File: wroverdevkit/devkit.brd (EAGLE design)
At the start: 33 x 59.4 mm, 42 parts, among them IC1 FT231XQ, Q3 BSS138, Q4 BSS138, T1 TRANSISTORMMBT2222, T2 TRANSISTORMMBT2222, T3 TRANSISTORMMBT2222

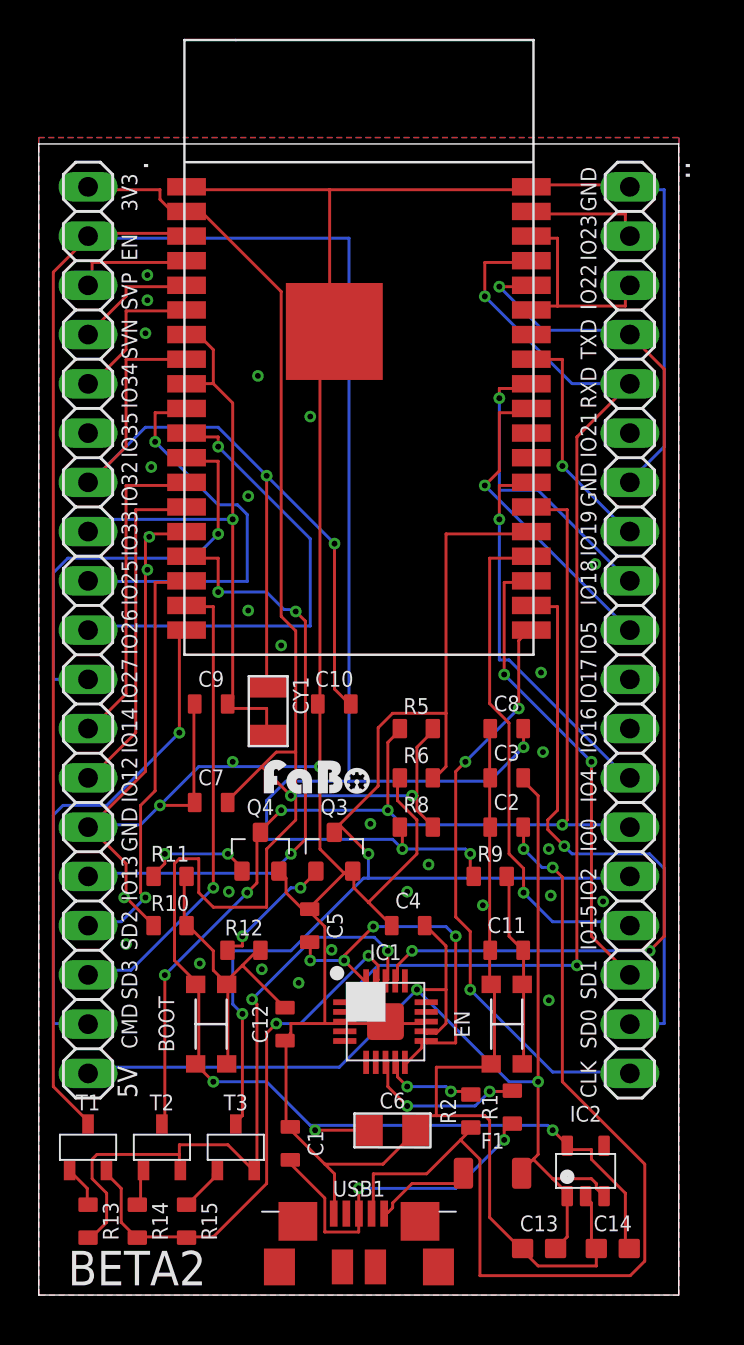
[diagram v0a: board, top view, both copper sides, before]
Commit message: devボード見直し
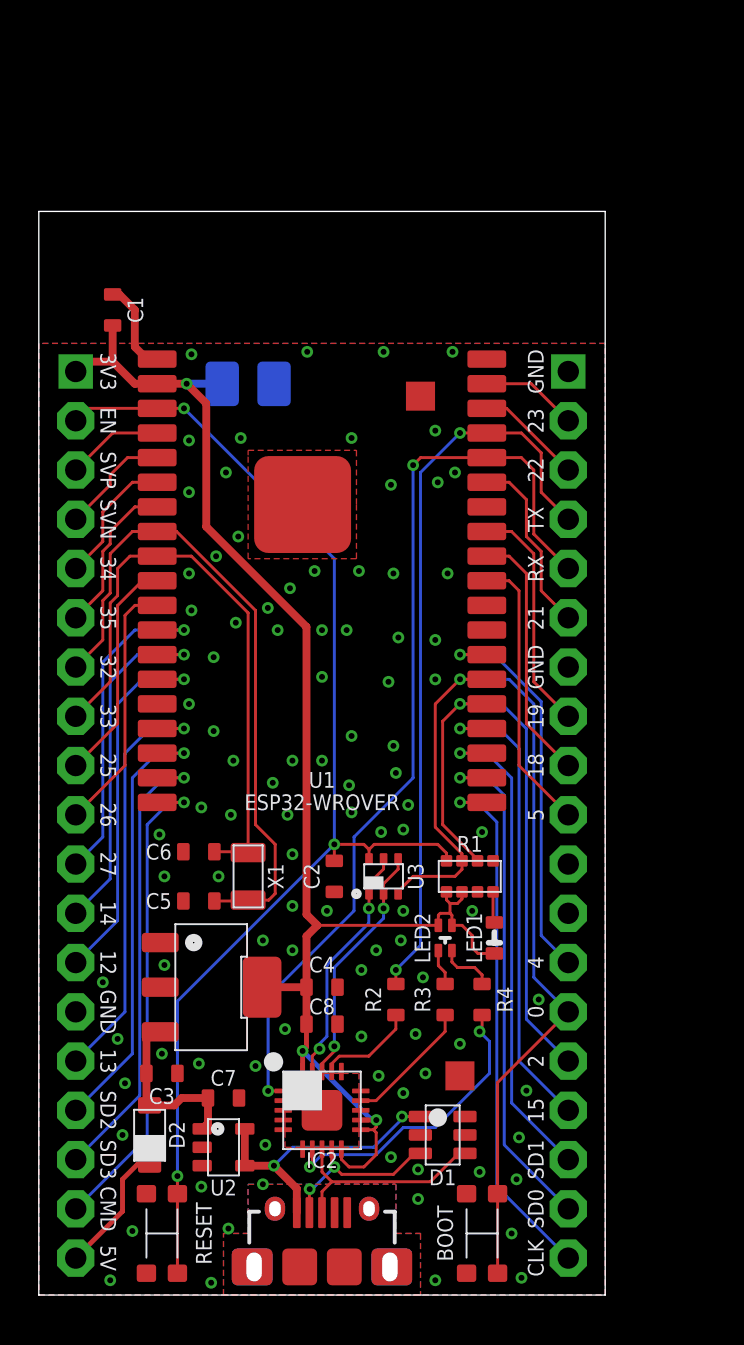
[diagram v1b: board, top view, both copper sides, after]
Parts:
- removed ., ..: (no value), pinhead:1X19
- removed C10, C9: 27pf, FaBo-Capacitor:0603-NARROW
- removed C11, C12: 1nf, FaBo-Capacitor:0603-NARROW
- removed C13, C14: 1uF, FaBo-Capacitor:0603
- removed CY1: CRYSTALABS07, FaBo-Crystal:ABRACOM-ABS07-32.768KHZ
- removed EN: (no value), FaBo-Switch:KMR2
- removed F1: (no value), FaBo-Parts:NANOSMDC035F
- removed Q3, Q4: BSS138, FaBo-etc:SOT23-3
- removed R10: 10K, FaBo-Resistors:0603-NARROW
- removed R11, R12: 1K, FaBo-Resistors:0603-NARROW
- removed R13, R14, R15: 100K, FaBo-Resistors:0603-NARROW
- removed R5, R6: 5K, FaBo-Resistors:0603-NARROW
- removed R8: 12K, FaBo-Resistors:0603-NARROW
- removed R9: 470, FaBo-Resistors:0603-NARROW
- removed T1, T2, T3: TRANSISTORMMBT2222, FaBo-Transistor:SOT-23
- removed U$1: ESP32-WROVER, FaBo-ESP32:ESP32-WROVER
- removed U$3: (no value), FaBo-Logo:LOGO_FABO_S
- added C0: NP, component:MULTIPAD0603
- added CN1, CN2: (no value), component:PIN_1X19
- added D1: ESDA6V1BC6, component:SOT-23-6L
- added D2: (no value), component:SOD-123FL_RB161MM-20
- added FID1, FID2: FIDUCIAL-TOP, component:FIDUCIAL_15_TOP
- added LED1: (no value), component:LED_0603
- added LED2: (no value), component:HSMF-C16X
- added LOGO1: (no value), component:LOGO_FABO_M_BOTTOM
- added R3, R4: 1k, component:EIA0603
- added RESET: (no value), component:KMR2-TACT
- added U1: (no value), component:ESP32-WROVER-B
- added U2: TPS2065DBVR, component:SOT-23-5
- added U3: BS138PS, component:SOT-363
- added X1: 32.768k, component:ABS07
- BOOT: device FaBo-Switch:KMR2 -> component:KMR2-TACT
- C1: value 47pF -> 0.1uF; device FaBo-Capacitor:0603-NARROW -> component:EIA0603
- C2: value 47pF -> 0.01uF; device FaBo-Capacitor:0603-NARROW -> component:EIA0603
- C3: value 0.1uF -> 1uF; device FaBo-Capacitor:0603-NARROW -> component:EIA0603
- C4: value 4.7uF -> 1uF; device FaBo-Capacitor:0603-NARROW -> component:EIA0603
- C5: value 0.1uF -> 4.3pF; device FaBo-Capacitor:0603-NARROW -> component:EIA0603
- C6: value 100uF -> 4.3pF; device FaBo-Capacitor:1206 -> component:EIA0603
- C7: value 1uf -> 10uF; device FaBo-Capacitor:0603-NARROW -> component:EIA0603
- C8: value 0.1uf -> 0.1uF; device FaBo-Capacitor:0603-NARROW -> component:EIA0603
- IC1: value FT231XQ -> ADP3338AKCZ-3.3; device FaBo-USB:QFN-20_FT231X -> component:SOT-223-KC3
- IC2: value (none) -> FT231XQ; device FaBo-Supply:SOT-23-5 -> component:QFN-20
- R1: value 27 -> 10k; device FaBo-Resistors:0603-NARROW -> component:EXBV8V
- R2: value 27 -> 470; device FaBo-Resistors:0603-NARROW -> component:EIA0603
- USB1: value (none) -> ZX62D-B-5PA8(30); device FaBo-USB:ZX62R-B-5P -> component:ZX62D-B-5PA8
- moved C1 43.9 mm to (3.81, 50.8)
- moved C3 23.4 mm to (6.35, 11.4), turned to 180 degrees
- moved C8 18.0 mm to (14.6, 14.0), turned to 180 degrees
- moved BOOT 17.7 mm to (22.9, 3.17)
- moved C6 17.5 mm to (8.26, 22.9)
- moved C7 15.3 mm to (9.53, 10.2), turned to 180 degrees
- moved IC2 13.9 mm to (14.6, 9.53)
- moved R1 12.1 mm to (22.2, 21.6), turned to 0 degrees
- moved C2 9.25 mm to (15.2, 21.6), turned to 90 degrees
- moved IC1 9.16 mm to (8.89, 15.9), turned to 270 degrees
- moved R2 6.93 mm to (18.4, 15.2)
- moved C5 5.85 mm to (8.26, 20.3), turned to 0 degrees
- moved C4 5.46 mm to (14.6, 15.9), turned to 180 degrees
- moved USB1 1.91 mm to (14.6, 0.00)
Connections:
- removed net CBUS1: IC1.14
- removed net CBUS2: IC1.7
- removed net IO16: ...12
- removed net IO17: ...11
- removed net N$1: R13.1, T1.1
- removed net N$11: Q4.1, R11.1
- removed net N$12: Q3.1, R12.1
- removed net N$2: R14.1, T2.1
- removed net N$29: U$1.P$32
- removed net N$3: C2.2, R2.1, USB1.2
- removed net N$34: U$1.P$28
- removed net N$36: U$1.P$27
- removed net N$4: C1.2, R1.1, USB1.3
- removed net N$5: C11.2, EN.3, EN.4, R9.2
- removed net N$6: BOOT.3, BOOT.4, C12.2, R10.2, R11.2, R12.2
- removed net N$7: C5.2, IC1.10, IC1.11, IC1.20
- removed net N$8: R15.1, T3.1
- removed net SVN: ..4, U$1.P$5
- removed net SVP: ..3, U$1.P$4
- removed net VBUS: F1.1, USB1.1
- new net LED1K: LED1.K, R1.4
- new net LED2K1: LED2.4, R3.2
- new net LED2K2: LED2.3, R4.2
- new net OUT5V: CN1.19, D2.K
- new net RXLED: IC2.14, R3.1
- new net SENSOR_VN: CN1.4, U1.5
- new net SENSOR_VP: CN1.3, U1.4
- new net TXLED: IC2.7, R4.1
- new net TXPIN: IC2.17, R2.1
- new net USBVBUS: D1.1, U2.4, U2.5, USB1.1
- net 3V3: now also C0.2, C1.2, C4.2, C8.2, CN1.1, IC1.4, IC2.10, IC2.11, IC2.12, IC2.20, LED1.A, LED2.1, LED2.2, R1.1, R1.2, U1.2; no longer ..1, BOOT.1, BOOT.2, C14.2, C6.-, C7.2, IC2.5, R5.2, R8.2, U$1.P$2
- net 5V: now also C7.2, D2.A, IC1.3, U2.1; no longer ..19, C13.2, C4.2, F1.2, IC1.12, IC2.1, IC2.3
- net CLK: now also CN2.19, U1.20; no longer ...19, U$1.P$20
- net CMD: now also CN1.18, U1.19; no longer ..18, U$1.P$19
- net DTR: now also IC2.18, U3.2, U3.4; no longer IC1.18, R13.2, T2.2, T3.2
- net EN: now also C2.2, CN1.2, R1.8, RESET.3, RESET.4, U1.3, U3.6; no longer ..2, C8.2, R8.1, R9.1, T1.3, U$1.P$3
- net GND: now also BOOT.1, BOOT.2, C0.1, C6.1, CN1.14, CN2.1, CN2.7, D1.2, D1.5, IC1.1, IC2.13, IC2.21, IC2.3, R1.3, R1.5, RESET.1, RESET.2, U1.1, U1.15, U1.38, U1.39, U2.2, USB1.B1, USB1.B2, USB1.B3, USB1.B4, USB1.T1, USB1.T2, USB1.T3, USB1.T4, USB1.T5, USB1.T6; no longer ...1, ...7, ..14, C10.1, C11.1, C12.1, C13.1, C14.1, C6.+, C9.1, EN.1, EN.2, IC1.13, IC1.21, IC1.3, IC2.2, Q3.2, Q4.2, R10.1, R6.1, U$1.P$1, U$1.P$15, U$1.P$38, U$1.P$39
- net IO0: now also BOOT.3, BOOT.4, CN2.14, R1.7, U1.25, U3.3; no longer ...14, Q4.3, R5.1, T2.3, U$1.P$25
- net IO12: now also CN1.13, U1.14; no longer ..13, U$1.P$14
- net IO13: now also CN1.15, U1.16; no longer ..15, U$1.P$16
- net IO14: now also CN1.12, U1.13; no longer ..12, U$1.P$13
- net IO15: now also CN2.16, U1.23; no longer ...16, U$1.P$23
- net IO18: now also CN2.9, U1.30; no longer ...9, U$1.P$30
- net IO19: now also CN2.8, U1.31; no longer ...8, U$1.P$31
- net IO2: now also CN2.15, R1.6, U1.24; no longer ...15, Q3.3, R6.2, T3.3, U$1.P$24
- net IO21: now also CN2.6, U1.33; no longer ...6
- net IO22: now also CN2.3, U1.36; no longer ...3, U$1.P$33, U$1.P$36
- net IO23: now also CN2.2, U1.37; no longer ...2, U$1.P$37
- net IO25: now also CN1.9, U1.10; no longer ..9, U$1.P$10
- net IO26: now also CN1.10, U1.11; no longer ..10, U$1.P$11
- net IO27: now also CN1.11, U1.12; no longer ..11, U$1.P$12
- net IO32: now also C5.2, CN1.7, U1.8, X1.1; no longer ..7, C10.2, CY1.P$1, U$1.P$8
- net IO33: now also C6.2, CN1.8, U1.9, X1.2; no longer ..8, C9.2, CY1.P$2, U$1.P$7, U$1.P$9
- net IO34: now also CN1.5, U1.6; no longer ..5, U$1.P$6
- net IO35: now also CN1.6, U1.7; no longer ..6
- net IO4: now also CN2.13, U1.26; no longer ...13, U$1.P$26
- net IO5: now also CN2.10, U1.29; no longer ...10, U$1.P$29
- net RTS: now also IC2.19, U3.1, U3.5; no longer IC1.19, R14.2, R15.2, T1.2
- net RXD: now also CN2.5, IC2.1, U1.34; no longer ...4, IC1.17, U$1.P$34
- net SD0: now also CN2.18, U1.21; no longer ...18, U$1.P$21
- net SD1: now also CN2.17, U1.22; no longer ...17, U$1.P$22
- net SD2: now also CN1.16, U1.17; no longer ..16, U$1.P$17
- net SD3: now also CN1.17, U1.18; no longer ..17, U$1.P$18
- net TXD: now also CN2.4, R2.2, U1.35; no longer ...5, IC1.1, U$1.P$35
- net USBDM: now also D1.3, IC2.9, USB1.2; no longer IC1.9, R2.2
- net USBDP: now also D1.4, IC2.8, USB1.3; no longer IC1.8, R1.2
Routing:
- net GND: track 213.0 -> 4.79 mm, vias 32 -> 98
- net EN: track 124.5 -> 64.9 mm
- net 5V: track 65.1 -> 9.22 mm, vias 2 -> 0
- net N$3: track 49.7 -> 0.00 mm, vias 2 -> 0
- net 3V3: track 113.5 -> 75.8 mm, vias 5 -> 3
- net IO2: track 62.6 -> 32.6 mm, vias 2 -> 1
- net DTR: track 34.4 -> 12.6 mm
- net N$7: track 19.9 -> 0.00 mm, vias 4 -> 0
- net TXD: track 57.8 -> 38.4 mm, vias 3 -> 2
- net N$4: track 18.0 -> 0.00 mm, vias 2 -> 0
- net N$6: track 16.3 -> 0.00 mm
- net RTS: track 28.2 -> 12.5 mm
- net TXLED: track 0.00 -> 15.5 mm, vias 0 -> 2
- net USBVBUS: track 0.00 -> 15.0 mm, vias 0 -> 2
- net IO26: track 25.0 -> 13.2 mm, vias 1 -> 0
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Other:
- board size 33 x 59.4 mm -> 29.2 x 55.9 mm
- board text added: "0"
- board text added: "12"
- board text added: "13"
- board text added: "14"
- board text added: "15"
- board text added: "18"
- board text added: "19"
- board text added: "2"
- board text added: "21"
- board text added: "22"
- board text added: "23"
- board text added: "25"
- board text added: "26"
- board text added: "27"
- board text added: "32"
- board text added: "33"
- board text added: "34"
- board text added: "35"
- board text added: "4"
- board text added: "5"
- board text added: "ESP32 WROVER DevBoard"
- board text added: "MADE IN JAPAN"
- board text added: "RX"
- board text added: "Rev.0.3"
- board text added: "TX"
- board text removed: "BETA2"
- board text removed: "IO0"
- board text removed: "IO12"
- board text removed: "IO13"
- board text removed: "IO14"
- board text removed: "IO15"
- board text removed: "IO16"
- board text removed: "IO17"
- board text removed: "IO18"
- board text removed: "IO19"
- board text removed: "IO2"
- board text removed: "IO21"
- board text removed: "IO22"
- board text removed: "IO23"
- board text removed: "IO25"
- board text removed: "IO26"
- board text removed: "IO27"
- board text removed: "IO32"
- board text removed: "IO33"
- board text removed: "IO34"
- board text removed: "IO35"
- board text removed: "IO4"
- board text removed: "IO5"
- board text removed: "RXD"
- board text removed: "TXD"
